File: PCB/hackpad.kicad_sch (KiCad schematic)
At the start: 27 parts, among them J1 Conn_01x04_Pin, SW1 RotaryEncoder_Switch, SW2 SW_Push, SW3 SW_Push, SW4 SW_Push, SW5 SW_Push, SW6 SW_Push, SW7 SW_Push, SW8 SW_Push, SW9 SW_Push, U1 XIAO-RP2040-DIP

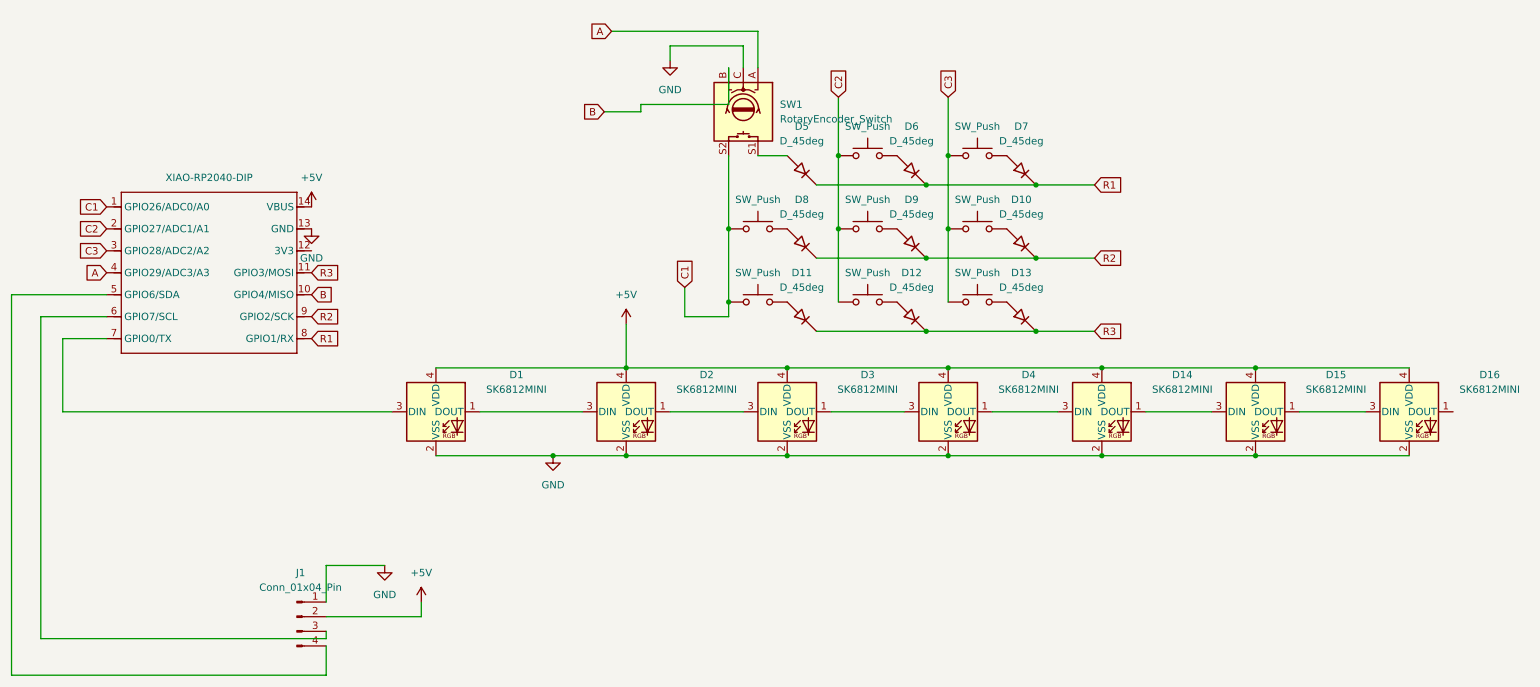
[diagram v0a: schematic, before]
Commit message: Update hackpad.kicad_sch
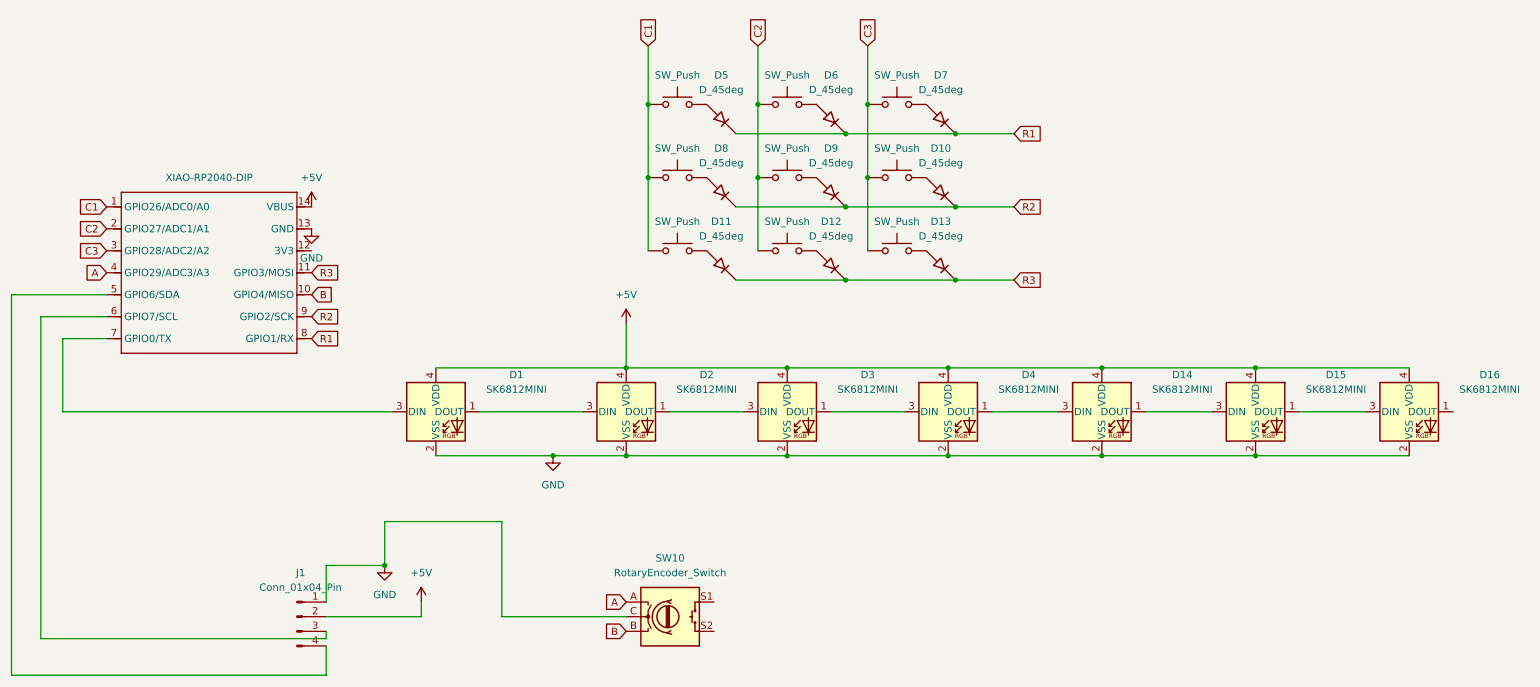
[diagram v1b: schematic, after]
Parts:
- removed SW1: RotaryEncoder_Switch, Rotary_Encoder:RotaryEncoder_Alps_EC11E-Switch_Vertical_H20mm_CircularMountingHoles, symbol Device:RotaryEncoder_Switch
- added SW1: SW_Push, Button_Switch_Keyboard:SW_Cherry_MX_1.00u_PCB, symbol Switch:SW_Push
- added SW10: RotaryEncoder_Switch, OLED:RotaryEncoder_Alps_EC11E_Vertical_H20mm, symbol Device:RotaryEncoder_Switch
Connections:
- net A: now also SW10.A
- net B: now also SW10.B
- net C1: now also SW1.1
- net GND: now also SW10.C
- net at D5.2 (A): now also SW1.2
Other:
- moved on the sheet: D10, D11, D12, D13, D5, D6, D7, D8, D9
